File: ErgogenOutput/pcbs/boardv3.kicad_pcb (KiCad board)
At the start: 2 copper layers, 167 x 122.9 mm, 91 parts

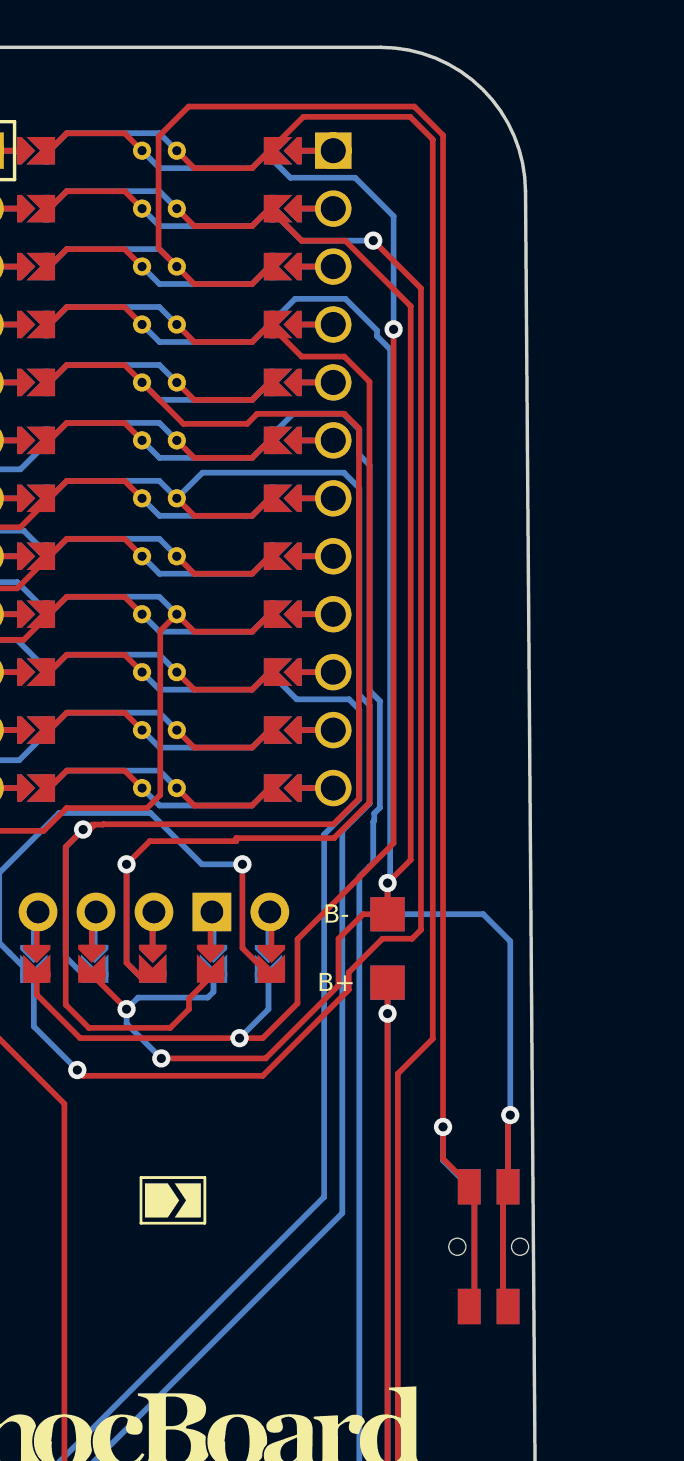
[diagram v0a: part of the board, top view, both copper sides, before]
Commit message: pnp
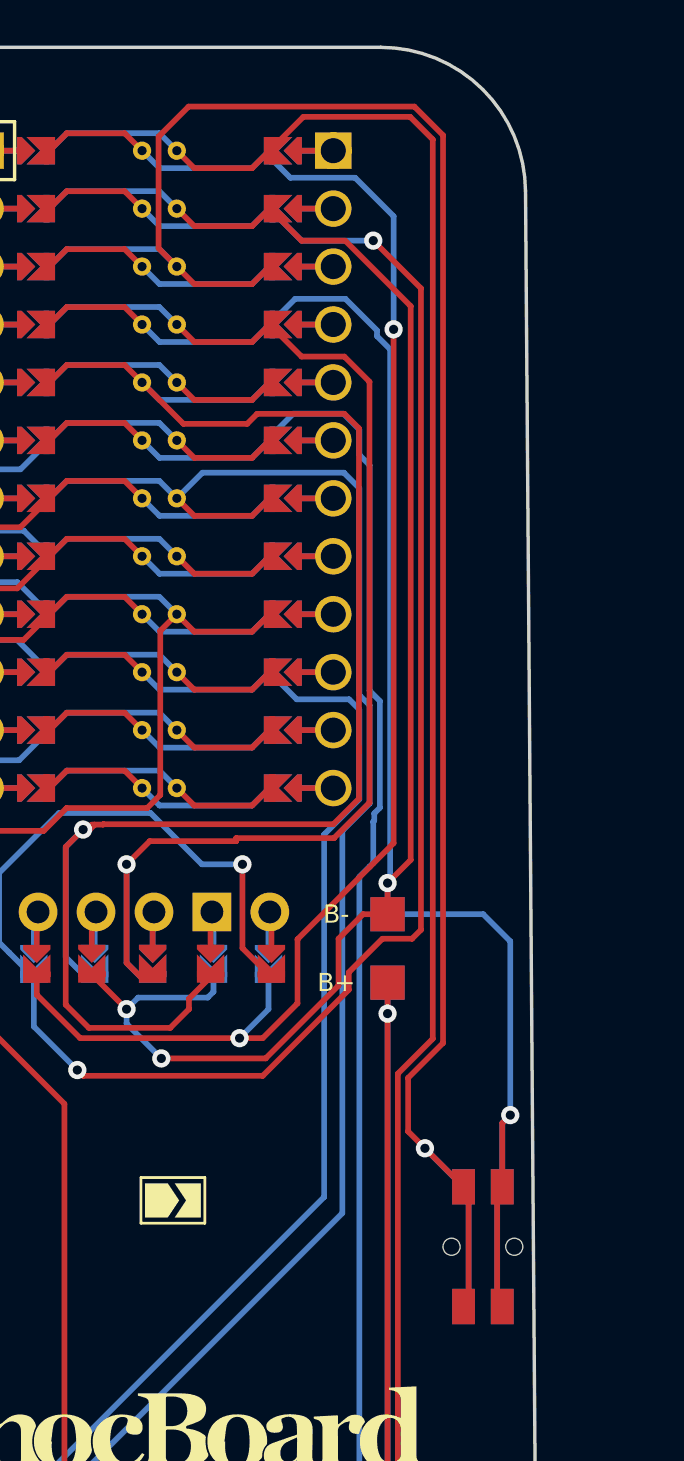
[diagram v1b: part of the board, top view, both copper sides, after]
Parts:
- moved ? 0.25 mm to (166.3, 71.7)
- moved ? 0.25 mm to (166.3, 76.9)
- moved REF** 0.25 mm to (165.5, 74.3)
- moved ? 0.25 mm to (164.6, 71.7)
- moved ? 0.25 mm to (164.6, 76.9)
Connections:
- REF** pad : (no net) -> RST
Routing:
- net RST: track 79.7 -> 81.0 mm
